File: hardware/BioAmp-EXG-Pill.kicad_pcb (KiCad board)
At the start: 2 copper layers, 25.4 x 10 mm, 30 parts, among them J1 Conn_01x03, J2 Conn_01x03, U1 TL074

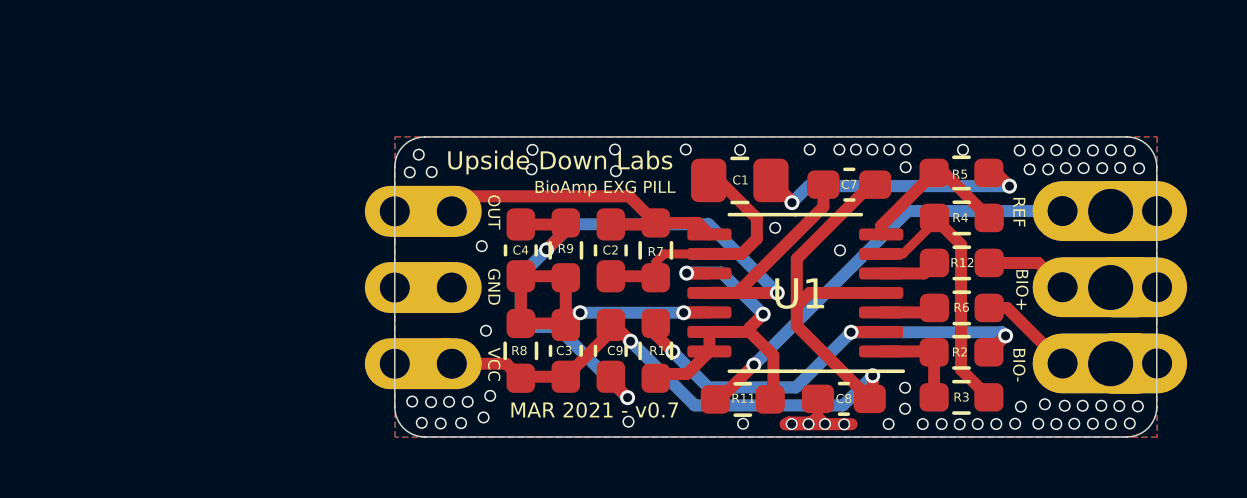
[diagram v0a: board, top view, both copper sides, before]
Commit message: BioAmp EXG Pill v0.9 KiCAD PCB
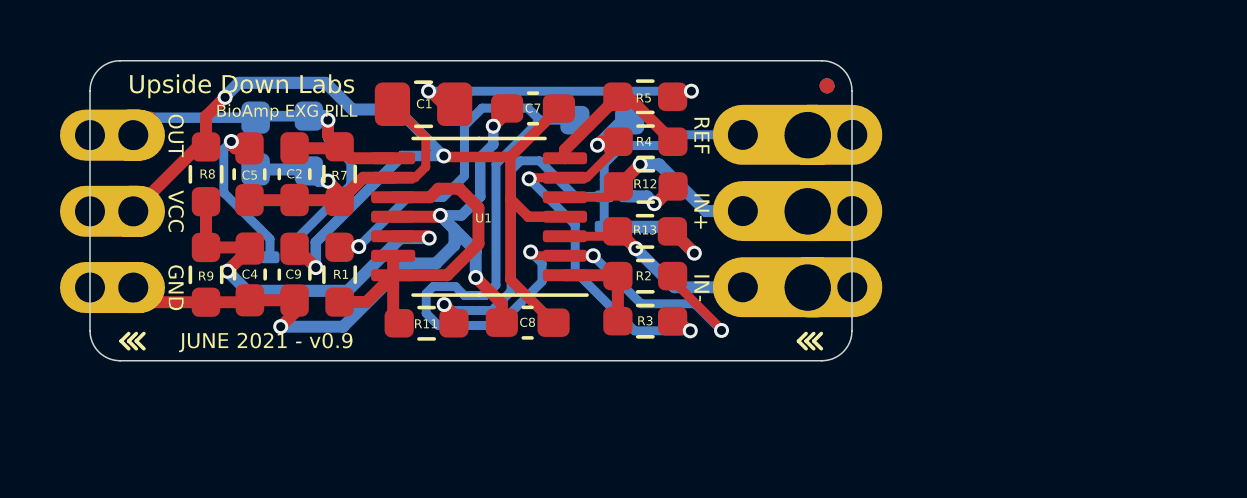
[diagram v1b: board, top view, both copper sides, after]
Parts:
- removed ? (x6): , buzzard_labels
- removed C3: 100n, Capacitor_SMD:C_0603_1608Metric_Pad1.08x0.95mm_HandSolder
- removed the G*** at (131.6, 97.0)
- added C2: 4.7nF, Capacitor_SMD:C_0603_1608Metric_Pad1.08x0.95mm_HandSolder, B.Cu at (116.5, 92.2)
- added C5: 47nF, Capacitor_SMD:C_0603_1608Metric_Pad1.08x0.95mm_HandSolder, F.Cu at (116.3, 93.2)
- added G***: LOGO, udlabs:EXG, B.Cu at (122.3, 94.4)
- added R10: 0R, Resistor_SMD:R_0201_0603Metric_Pad0.64x0.40mm_HandSolder, B.Cu at (117.3, 96.0)
- added R13: 1M, Resistor_SMD:R_0603_1608Metric_Pad0.98x0.95mm_HandSolder, F.Cu at (129.4, 95.1)
- added R14: 0R, Resistor_SMD:R_0201_0603Metric_Pad0.64x0.40mm_HandSolder, B.Cu at (128.5, 95.0)
- added R15: 0R, Resistor_SMD:R_0201_0603Metric_Pad0.64x0.40mm_HandSolder, B.Cu at (128.5, 94.0)
- added R7: 1M, Resistor_SMD:R_0603_1608Metric_Pad0.98x0.95mm_HandSolder, B.Cu at (118.2, 92.2)
- added REF**: Fiducial_0.5mm_Mask1mm, Fiducial:Fiducial_0.5mm_Mask1mm, B.Cu at (135.5, 90.3)
- added REF**: Fiducial_0.5mm_Mask1mm, Fiducial:Fiducial_0.5mm_Mask1mm, F.Cu at (135.5, 90.3)
- C1: value 47uf -> 47uF
- C2: value 100pf -> 4.7nF
- C4: value 100n -> 2.2uF
- C7, C9: value 100nf -> 100nF
- C8: value 2.2uf -> 2.2uF
- J1 (x2): value Conn_01x03 -> BioAmp Input
- J2 (x2): value Conn_01x03 -> BioAmp Output
- R1, R4, R8, R9: value 10k -> 10K
- R11: value 100k -> 1k
- R12: value 100k -> 1M
- R2, R3, R5: value 1k -> 1K
- R6: value 100k -> RG; moved to B.Cu
- moved R6 13.5 mm to (128.0, 91.4), turned to 180 degrees
- moved R8 12.0 mm to (114.8, 93.2), turned to 90 degrees
- moved R9 12.0 mm to (114.8, 96.6), turned to 90 degrees
- moved J1 11.0 mm to (132.7, 91.9)
- moved J2 10.9 mm to (112.4, 91.9)
- moved C2 10.8 mm to (117.8, 93.2)
- moved R7 10.8 mm to (119.3, 93.2)
- moved C9 10.8 mm to (117.8, 96.6)
- moved R1 10.8 mm to (119.3, 96.6)
- moved C1 10.8 mm to (122.1, 90.9)
- moved C7 10.8 mm to (125.7, 91.0), turned to 0 degrees
- moved C8 10.8 mm to (125.5, 98.2)
- moved R2 10.8 mm to (129.4, 96.6)
- moved R3 10.8 mm to (129.4, 98.1)
- moved R4 10.8 mm to (129.5, 92.2)
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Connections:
- net vRef renamed Net-(C4-Pad1)
- C7 pad 1: VCC -> GND
- C7 pad 2: GND -> VCC
- J1 pad 2: BIO+ -> IN+ (x2)
- J1 pad 3: BIO- -> IN- (x2)
- J2 pad 2: GND -> VCC (x2)
- J2 pad 3: VCC -> GND (x2)
- R12 pad 2: BIO+ -> IN+
- R6 pad 1: Net-(R6-Pad1) -> Net-(R3-Pad1)
- R6 pad 2: BIO- -> Net-(R1-Pad1)
- U1 pad 3: Net-(R6-Pad1) -> IN-
- U1 pad 5: Net-(R12-Pad1) -> IN+
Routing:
- net Net-(R1-Pad1): track 15.3 -> 36.2 mm, vias 3 -> 4
- net GND: track 35.9 -> 25.0 mm, vias 75 -> 4
- net OUT: track 11.2 -> 19.6 mm, vias 0 -> 1
- net IN+: track 0.00 -> 7.03 mm, vias 0 -> 2
- net IN-: track 0.00 -> 6.77 mm, vias 0 -> 2
- net Net-(R3-Pad1): track 9.09 -> 14.8 mm, vias 0 -> 3
- net Net-(C5-Pad1): track 0.00 -> 5.58 mm, vias 0 -> 1
- net BIO-: track 5.31 -> 0.00 mm, vias 1 -> 0
- net DRL: track 14.3 -> 18.2 mm
- net Net-(C1-Pad1): track 8.57 -> 12.3 mm, vias 0 -> 1
- net Net-(R13-Pad1): track 0.00 -> 3.59 mm, vias 0 -> 1
- net VCC: track 30.7 -> 33.7 mm, vias 2 -> 3
- net BIO+: track 2.87 -> 0.00 mm, vias 1 -> 0
- net Net-(R6-Pad1): track 1.84 -> 0.00 mm
- net Net-(C4-Pad1): track 11.4 -> 13.0 mm
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- removed copper zone on B.Cu, net GND
- removed copper zone on F.Cu, net GND
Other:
- board text added: "2E"
- board text added: "3E"
- board text added: "BioAmp EXG Pill"
- board text added: "EMG"
- board text added: "EXG"
- board text added: "FILTER"
- board text added: "GAIN"
- board text added: "IN+"
- board text added: "IN-"
- board text added: "INPUT"
- board text added: "JUNE 2021 - v0.9"
- board text added: "SIGNAL"
- board text added: "v0.9"
- board text removed: "BIO+"
- board text removed: "BIO-"
- board text removed: "BioAmp EXG Pill v0.7"
- board text removed: "MAR 2021 - v0.7"

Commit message: Update v0.9 PCB silk screen
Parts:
- C2 (x2): value 4.7nF -> 47nF
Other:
- board text added: "BandPass"
- board text added: "ELECTRODES"
- board text added: "WIDE"
- board text removed: "EMG"
- board text removed: "EXG"
- board text removed: "INPUT"
- board text removed: "SIGNAL"
